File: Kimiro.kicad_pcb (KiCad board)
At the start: 2 copper layers, 17.8 x 33 mm, 29 parts, among them J1 Conn_01x04, J2 USB_C_Left, J3 Left, J4 Right, U2 BQ24075/9, U3 MS88FS3, U4 XC6220B331MR

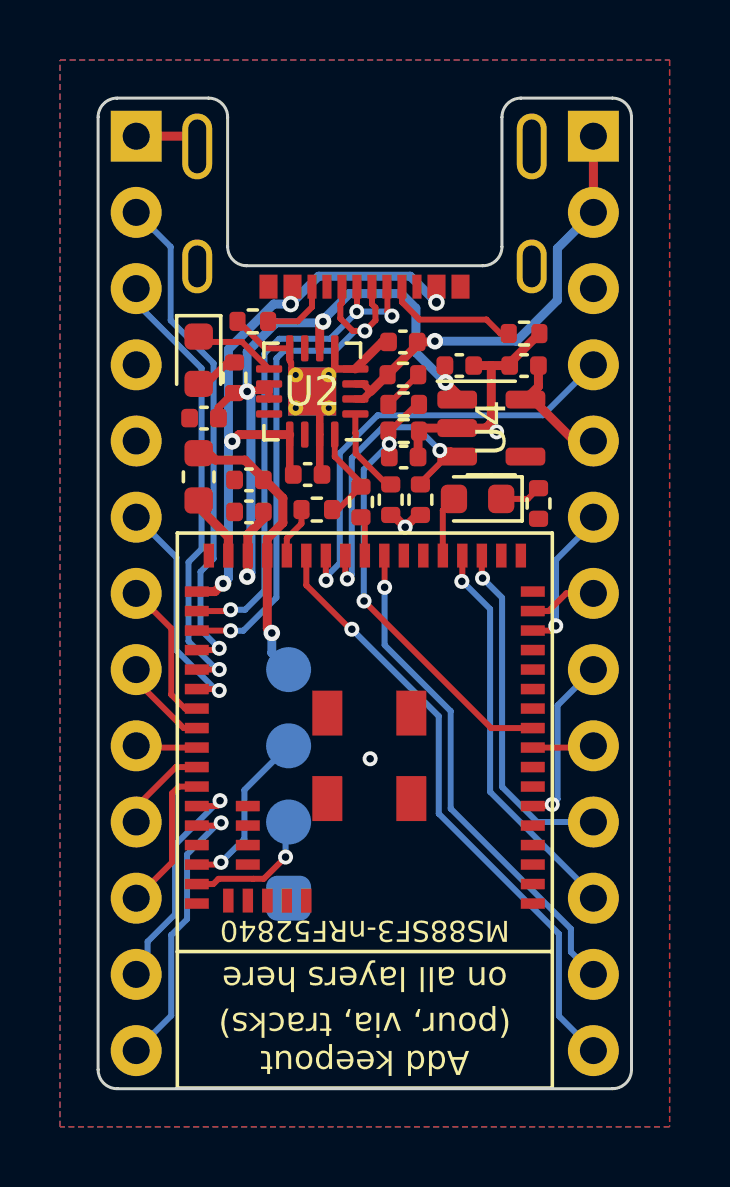
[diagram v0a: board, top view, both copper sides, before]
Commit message: 20:00 15/03/2022
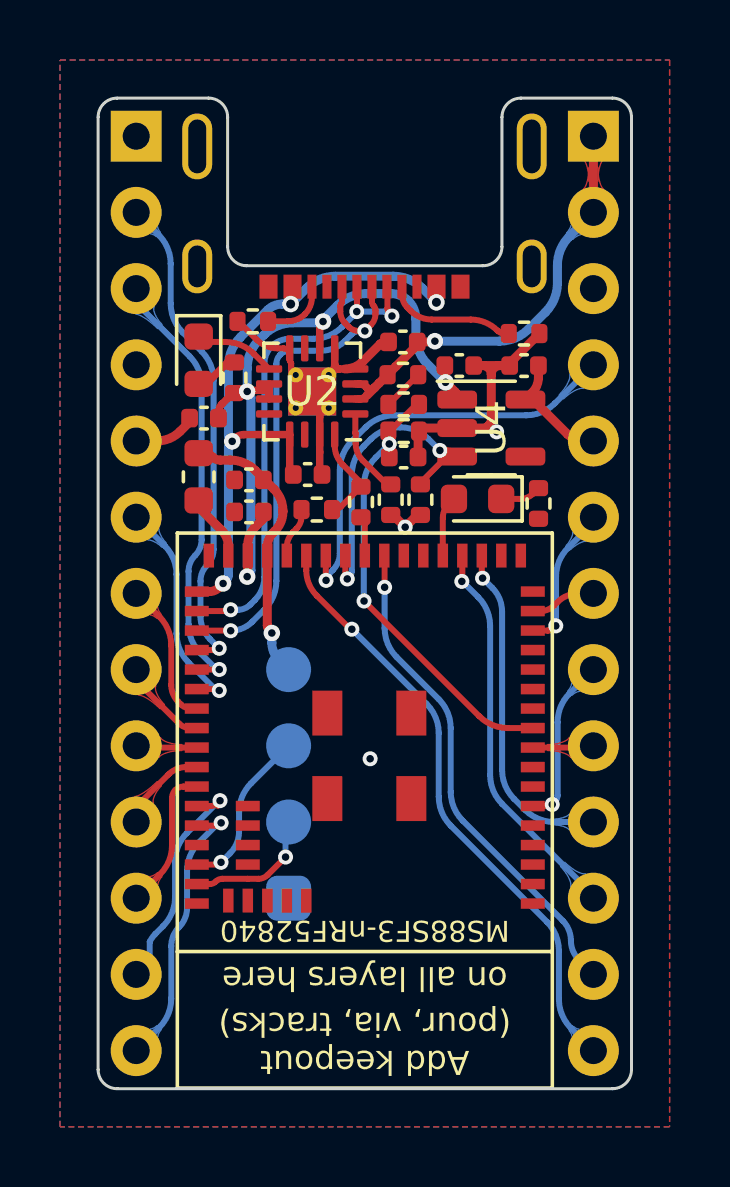
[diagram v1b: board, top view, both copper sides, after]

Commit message: cập nhật PCB
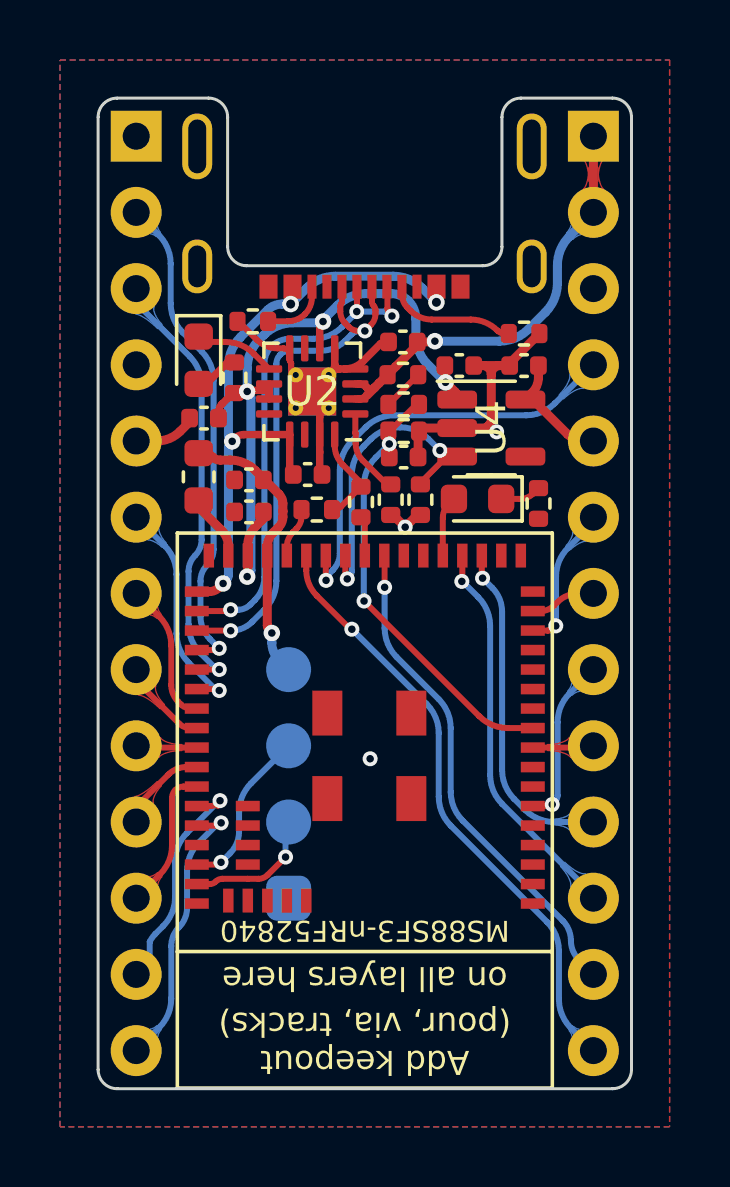
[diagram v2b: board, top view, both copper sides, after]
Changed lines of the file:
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@@
   (segment (start 70.041799 44.131199) (end 70.316617 43.856382) (width 0.3) (layer "F.Cu") (net 2))
   (segment (start 71.8592 45.7454) (end 71.75808 45.64428) (width 0.3) (layer "F.Cu") (net 2))
-  (segment (start 76.88795 41.148) (end 76.99 41.148) (width 0.3) (layer "F.Cu") (net 2))
   (segment (start 74.6974 43.650714) (end 74.6974 44.822286) (width 0.25) (layer "F.Cu") (net 2))
   (segment (start 71.8846 46.8122) (end 71.8846 46.854485) (width 0.3) (layer "F.Cu") (net 2))
-  (segment (start 76.127967 41.805931) (end 76.713739 41.22016) (width 0.3) (layer "F.Cu") (net 2))
+  (segment (start 76.127967 41.805931) (end 76.713739 41.22016) (width 0.25) (layer "F.Cu") (net 2))
   (segment (start 70.3606 43.7502) (end 70.3606 43.688) (width 0.3) (layer "F.Cu") (net 2))
   (segment (start 74.5724 42.924) (end 74.4474 42.799) (width 0.25) (layer "F.Cu") (net 2))
@@
   (arc (start 73.74692 41.992114) (mid 73.766474 42.09042) (end 73.82216 42.17376) (width 0.2) (layer "F.Cu") (net 2))
   (arc (start 79.259525 44.0182) (mid 79.266939 44.013245) (end 79.2652 44.0045) (width 0.3) (layer "F.Cu") (net 2))
-  (arc (start 76.127967 41.805931) (mid 75.858733 41.985828) (end 75.54115 42.049) (width 0.3) (layer "F.Cu") (net 2))
+  (arc (start 76.127967 41.805931) (mid 75.858733 41.985828) (end 75.54115 42.049) (width 0.25) (layer "F.Cu") (net 2))
   (arc (start 75.0974 42.149) (mid 75.17141 42.038234) (end 75.1974 41.907578) (width 0.25) (layer "F.Cu") (net 2))
   (arc (start 77.977 46.9158) (mid 77.952609 46.920651) (end 77.931932 46.934467) (width 0.3) (layer "F.Cu") (net 2))
@@
   (arc (start 81.055752 41.831447) (mid 81.035656 41.861523) (end 81.0286 41.897) (width 0.3) (layer "F.Cu") (net 2))
   (arc (start 71.999386 40.47348) (mid 71.986891 40.465131) (end 71.972153 40.4622) (width 0.2) (layer "F.Cu") (net 2))
-  (arc (start 76.88795 41.148) (mid 76.793667 41.166753) (end 76.713739 41.22016) (width 0.3) (layer "F.Cu") (net 2))
+  (arc (start 76.88795 41.148) (mid 76.793667 41.166753) (end 76.713739 41.22016) (width 0.25) (layer "F.Cu") (net 2))
   (arc (start 79.2652 44.0045) (mid 79.280374 44.014639) (end 79.298274 44.0182) (width 0.3) (layer "F.Cu") (net 2))
   (arc (start 72.601029 41.075123) (mid 72.918234 41.287073) (end 73.292403 41.3615) (width 0.2) (layer "F.Cu") (net 2))
@@
   (segment (start 75.55 48.935072) (end 75.55 48.269) (width 0.2) (layer "F.Cu") (net 15))
   (segment (start 75.6158 49.0474) (end 75.5829 49.0145) (width 0.2) (layer "F.Cu") (net 15))
+  (segment (start 79.2789 44.9682) (end 78.930999 44.9682) (width 0.2) (layer "F.Cu") (net 15))
   (segment (start 78.807998 45.091201) (end 78.0034 45.8958) (width 0.2) (layer "F.Cu") (net 15))
-  (segment (start 78.93086 44.764323) (end 78.702854 44.764323) (width 0.2) (layer "F.Cu") (net 15))
   (segment (start 79.10495 44.9682) (end 79.134737 44.9682) (width 0.2) (layer "F.Cu") (net 15))
+  (segment (start 78.930999 44.9682) (end 78.807998 45.091201) (width 0.2) (layer "F.Cu") (net 15))
   (via (at 78.702854 44.764323) (size 0.5) (drill 0.25) (layers "F.Cu" "B.Cu") (net 15))
   (via (at 75.6158 49.0474) (size 0.5) (drill 0.25) (layers "F.Cu" "B.Cu") (net 15))
   (arc (start 79.176961 44.866261) (mid 79.189905 44.931337) (end 79.134737 44.9682) (width 0.2) (layer "F.Cu") (net 15))
-  (arc (start 79.176961 44.866261) (mid 79.064049 44.790815) (end 78.93086 44.764323) (width 0.2) (layer "F.Cu") (net 15))
   (arc (start 75.55 48.935072) (mid 75.55855 48.978058) (end 75.5829 49.0145) (width 0.2) (layer "F.Cu") (net 15))
   (arc (start 79.10495 44.9682) (mid 78.94424 45.000166) (end 78.807998 45.091201) (width 0.2) (layer "F.Cu") (net 15))
@@
   (segment (start 71.384817 45.08588) (end 71.712222 45.08588) (width 0.3) (layer "F.Cu") (net 44))
   (segment (start 72.95 47.9845) (end 72.95 48.5535) (width 0.3) (layer "F.Cu") (net 44))
+  (segment (start 73.47028 46.766957) (end 73.470279 46.535966) (width 0.3) (layer "F.Cu") (net 44))
   (segment (start 73.0256 50.7752) (end 73.1012 50.8508) (width 0.3) (layer "F.Cu") (net 44))
   (segment (start 70.830562 44.8563) (end 70.6628 44.8563) (width 0.3) (layer "F.Cu") (net 44))
-  (segment (start 72.548265 45.43218) (end 73.178412 46.062327) (width 0.3) (layer "F.Cu") (net 44))
-  (segment (start 73.210139 47.439859) (end 73.151171 47.498828) (width 0.3) (layer "F.Cu") (net 44))
+  (segment (start 73.47028 46.811826) (end 73.47028 46.982253) (width 0.3) (layer "F.Cu") (net 44))
+  (segment (start 72.548265 45.43218) (end 73.341746 46.225661) (width 0.3) (layer "F.Cu") (net 44))
+  (segment (start 73.330654 47.319342) (end 73.151171 47.498828) (width 0.3) (layer "F.Cu") (net 44))
   (segment (start 73.47028 46.811826) (end 73.47028 46.766957) (width 0.3) (layer "F.Cu") (net 44))
   (segment (start 72.95 50.592685) (end 72.95 48.5535) (width 0.3) (layer "F.Cu") (net 44))
   (via (at 73.1012 50.8508) (size 0.55) (drill 0.25) (layers "F.Cu" "B.Cu") (net 44))
   (arc (start 73.151171 47.498828) (mid 73.002282 47.721656) (end 72.95 47.9845) (width 0.3) (layer "F.Cu") (net 44))
-  (arc (start 73.178412 46.062327) (mid 73.394425 46.385614) (end 73.47028 46.766957) (width 0.3) (layer "F.Cu") (net 44))
+  (arc (start 73.341746 46.225661) (mid 73.436874 46.36803) (end 73.470279 46.535966) (width 0.3) (layer "F.Cu") (net 44))
   (arc (start 71.10769 44.97109) (mid 71.234837 45.056047) (end 71.384817 45.08588) (width 0.3) (layer "F.Cu") (net 44))
   (arc (start 71.10769 44.97109) (mid 70.980542 44.886132) (end 70.830562 44.8563) (width 0.3) (layer "F.Cu") (net 44))
   (arc (start 72.548265 45.43218) (mid 72.164685 45.17588) (end 71.712222 45.08588) (width 0.3) (layer "F.Cu") (net 44))
-  (arc (start 73.47028 46.811826) (mid 73.402671 47.151715) (end 73.210139 47.439859) (width 0.3) (layer "F.Cu") (net 44))
+  (arc (start 73.47028 46.982253) (mid 73.433992 47.164684) (end 73.330654 47.319342) (width 0.3) (layer "F.Cu") (net 44))
   (arc (start 72.95 50.592685) (mid 72.969647 50.691461) (end 73.0256 50.7752) (width 0.3) (layer "F.Cu") (net 44))
   (segment (start 73.334686 51.744686) (end 73.66 52.07) (width 0.3) (layer "B.Cu") (net 44))
